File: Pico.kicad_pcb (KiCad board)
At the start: 2 copper layers, 36 parts, among them J1 DE15_Pins_HighDensity, J10 Conn_02x10_Odd_Even, J3 Conn_02x04_Odd_Even, J5 Micro_SD_Card, J8 W5500 Lite, U1 RASPBERRY_PI_PICO, U2 SN74LVC8T245, U4 74AHCT125, U6 RASPBERRY_PI_PICO

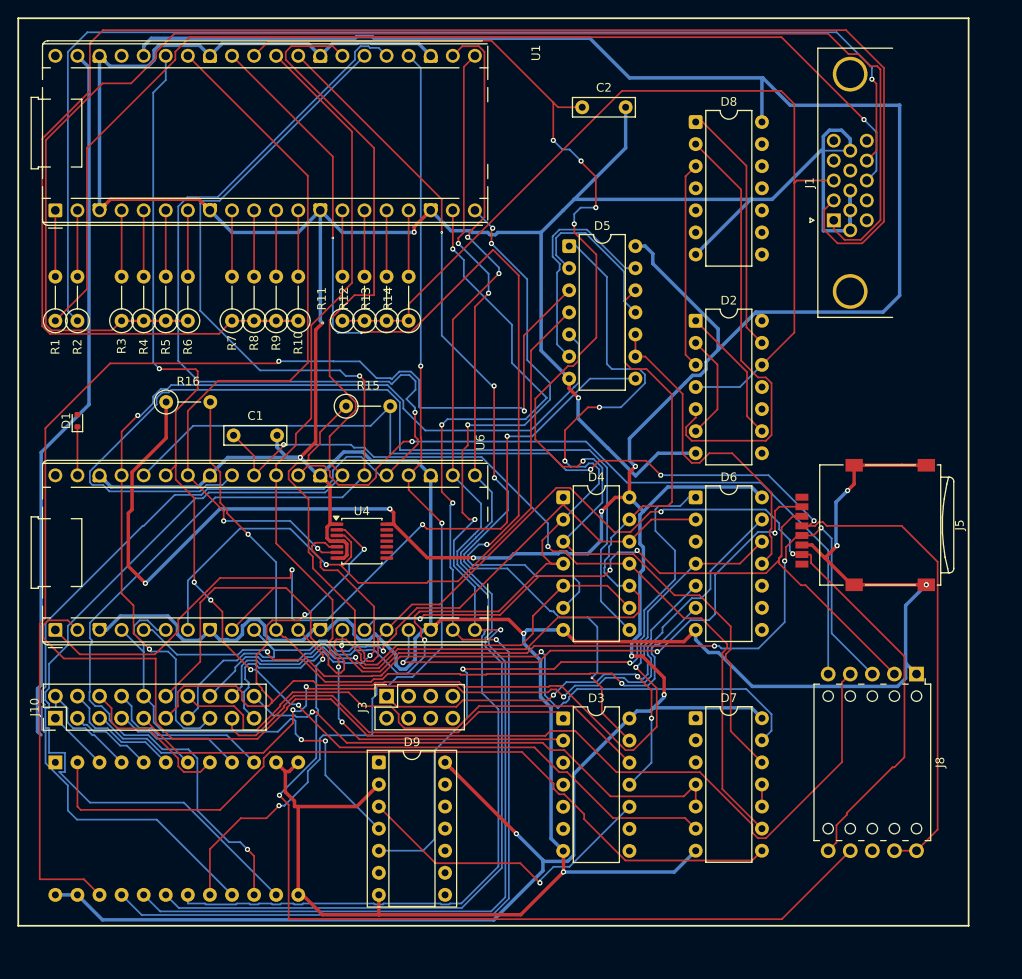
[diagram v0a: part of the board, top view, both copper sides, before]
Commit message: Fix PCB
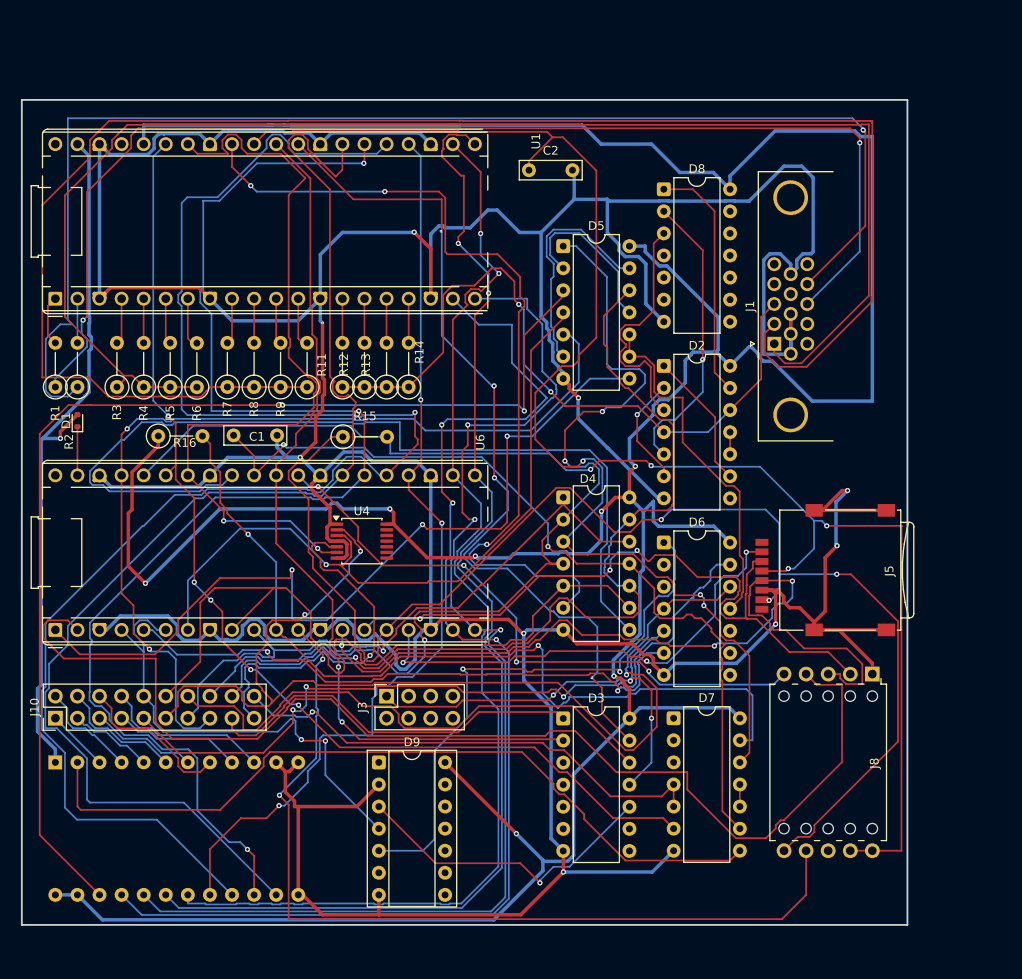
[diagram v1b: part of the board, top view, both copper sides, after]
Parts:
- moved J1 15.8 mm to (108.1, 68.7)
- moved U1 10.2 mm to (25.4, 63.5)
- moved C2 9.48 mm to (79.9, 48.7)
- moved D8 8.56 mm to (95.4, 50.9)
- moved R6 7.72 mm to (41.7, 73.7)
- moved R10 7.69 mm to (54.4, 73.7)
- moved R3 7.64 mm to (32.5, 73.7)
- moved R7 7.64 mm to (45.2, 73.7)
- moved R5 7.64 mm to (38.6, 73.7)
- moved R9 7.64 mm to (51.3, 73.7)
- moved R1 7.62 mm to (25.4, 73.7)
- moved R11 7.62 mm to (58.4, 73.7)
- moved R12 7.62 mm to (61.0, 73.7)
- moved R13 7.62 mm to (63.5, 73.7)
- moved R14 7.62 mm to (66.0, 73.7)
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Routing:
- net B: track 109.6 -> 82.3 mm, vias 0 -> 2
- net /~{CSW}: track 116.9 -> 98.0 mm
- net Net-(D2.2-B): track 51.4 -> 33.4 mm, vias 0 -> 1
- net /A1_33: track 140.8 -> 123.6 mm
- net /INT1: track 84.7 -> 70.4 mm, vias 1 -> 4
- net /CD3: track 146.7 -> 132.9 mm
- net /~{RES}: track 113.6 -> 100.4 mm
- net /CD7: track 157.6 -> 144.6 mm
- net /VSYNC: track 137.9 -> 150.8 mm
- net /HSYNC: track 128.6 -> 139.3 mm, vias 1 -> 2
- net /CD4: track 117.6 -> 107.4 mm
- net Net-(D5.1-Y): track 139.0 -> 129.1 mm
- net /~{RD}: track 84.0 -> 74.5 mm
- net /R: track 174.3 -> 165.9 mm
- net Net-(D6.1-A): track 74.0 -> 65.9 mm
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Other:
- board outline added: 101.9 x 94.9 mm

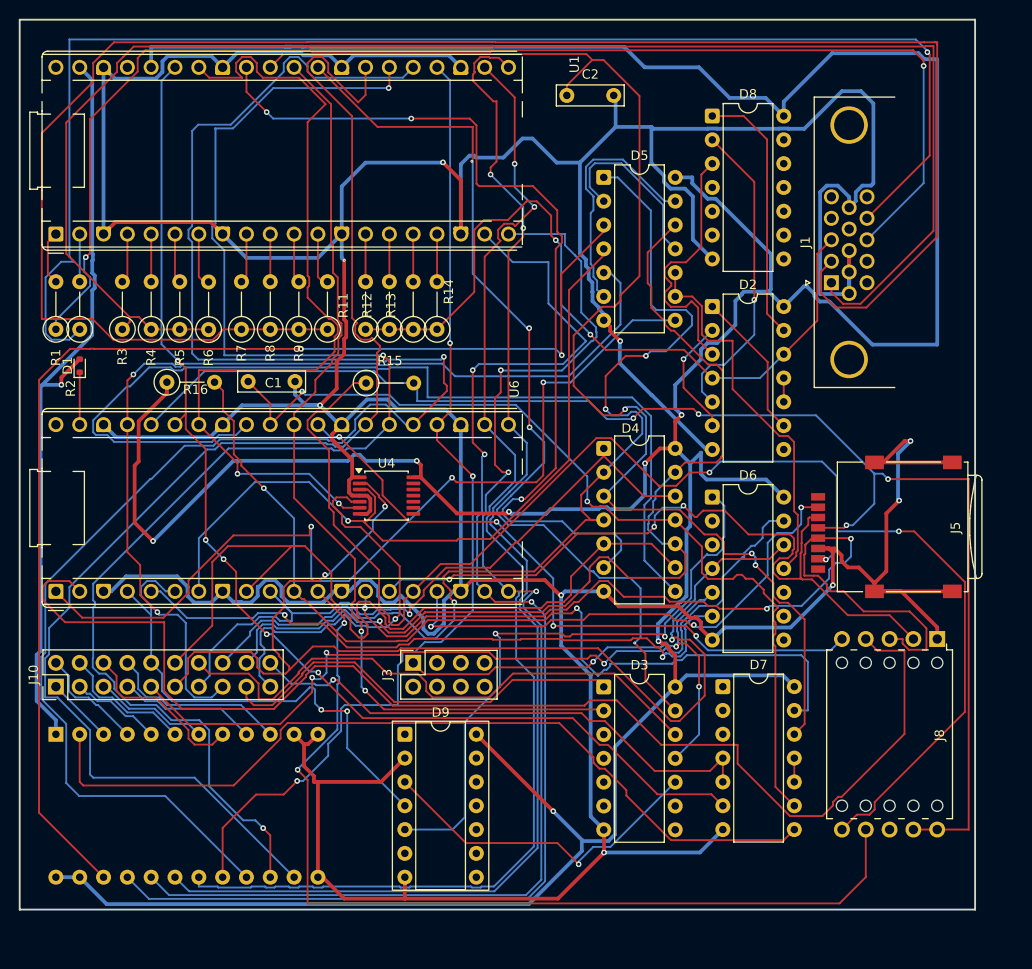
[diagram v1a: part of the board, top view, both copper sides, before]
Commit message: Fix PCB
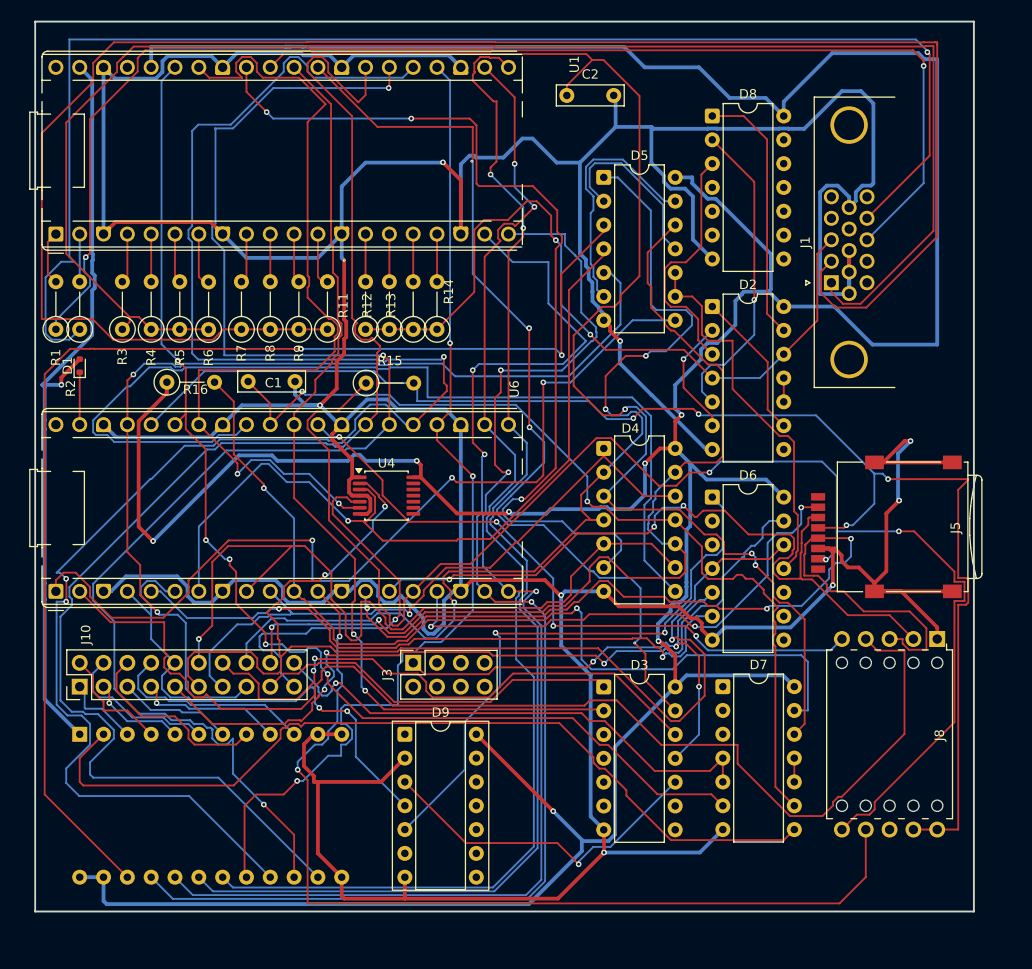
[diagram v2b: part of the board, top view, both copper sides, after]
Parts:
- moved J10 2.54 mm to (27.9, 111.8)
- moved U2 2.54 mm to (27.9, 116.8)
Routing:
- net /~{CS01}: track 134.7 -> 125.6 mm
- net /CD5: track 184.2 -> 190.1 mm, vias 1 -> 3
- net /RESET: track 44.6 -> 39.6 mm
- net +3V3: track 430.3 -> 425.5 mm
- net Net-(D6.1-A): track 65.9 -> 61.7 mm
- net /CD7: track 144.6 -> 148.8 mm
- net /CD3: track 132.9 -> 129.5 mm
- net /~{CS1}: track 107.5 -> 104.5 mm, vias 1 -> 2
- net /~{CS0}: track 112.5 -> 109.7 mm
- net /A1_33: track 123.6 -> 126.4 mm
- net /D7: track 19.3 -> 22.0 mm
- net /CD2: track 138.1 -> 135.6 mm
- net /CD1: track 135.5 -> 132.9 mm
- net /~{C100}: track 104.7 -> 107.2 mm
- net /CD0: track 138.4 -> 135.8 mm
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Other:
- board size 101.9 x 94.9 mm -> 100.1 x 94.9 mm
